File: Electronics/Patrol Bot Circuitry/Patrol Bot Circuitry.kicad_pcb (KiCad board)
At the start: 2 copper layers, 101 x 89.5 mm, 49 parts, among them J1 Left_Motor, J2 Right_Motor, J3 Battery, J4 AC_DC_10V, J5 Servo Motor, Q1 IRF4905, Q2 IRF4905, Q3 IRF4905, Q4 IRLZ44N, Q5 IRF4905, U1 ROB-14450, U10 HC-SR04, U11 MPU-6050, U2 ADS1115, U3 MP1584EN, U4 ESP32-CAM, U5 LM2931-3.3_TO220, U6 MAX9814, U7 MCP23017-E_SP, U8 HC-SR04, U9 HC-SR04

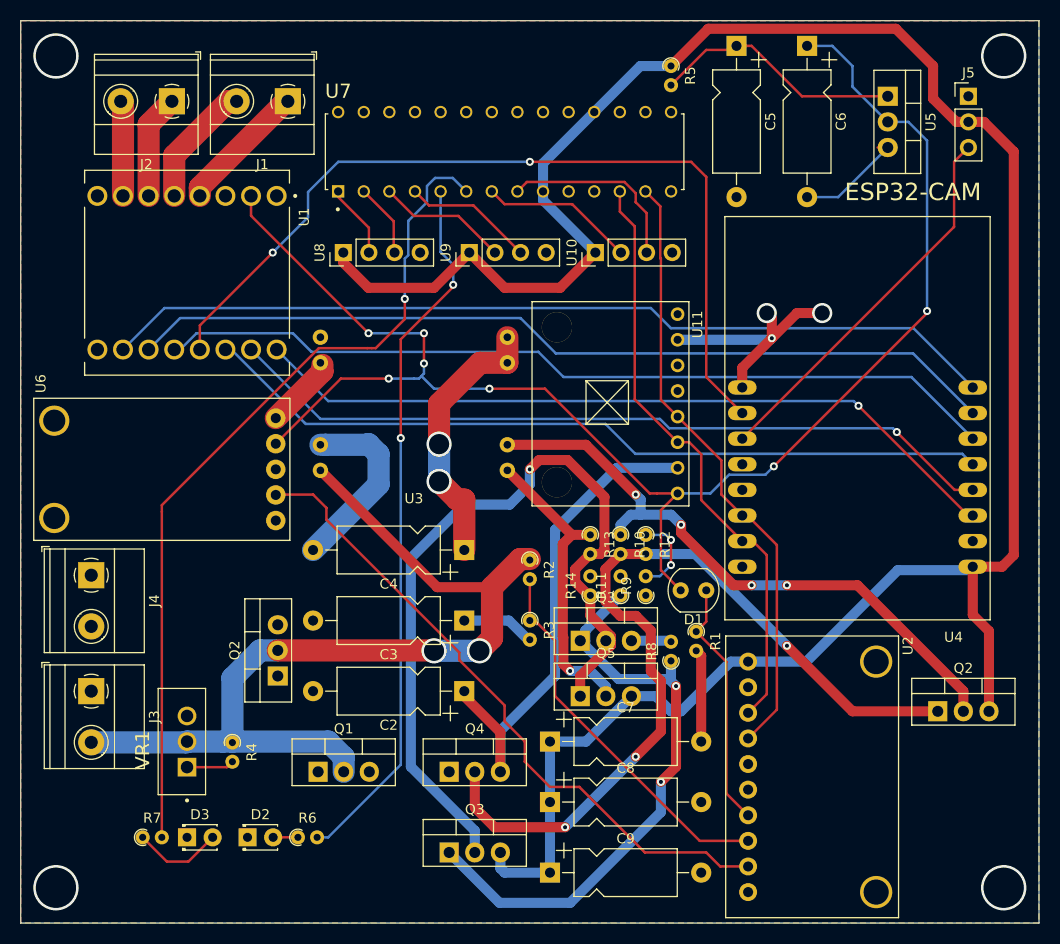
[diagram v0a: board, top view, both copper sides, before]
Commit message: Redesigned PCB / Mechanical Drawing
ESP32-cam not connecting to Wifi -> must DEBUG
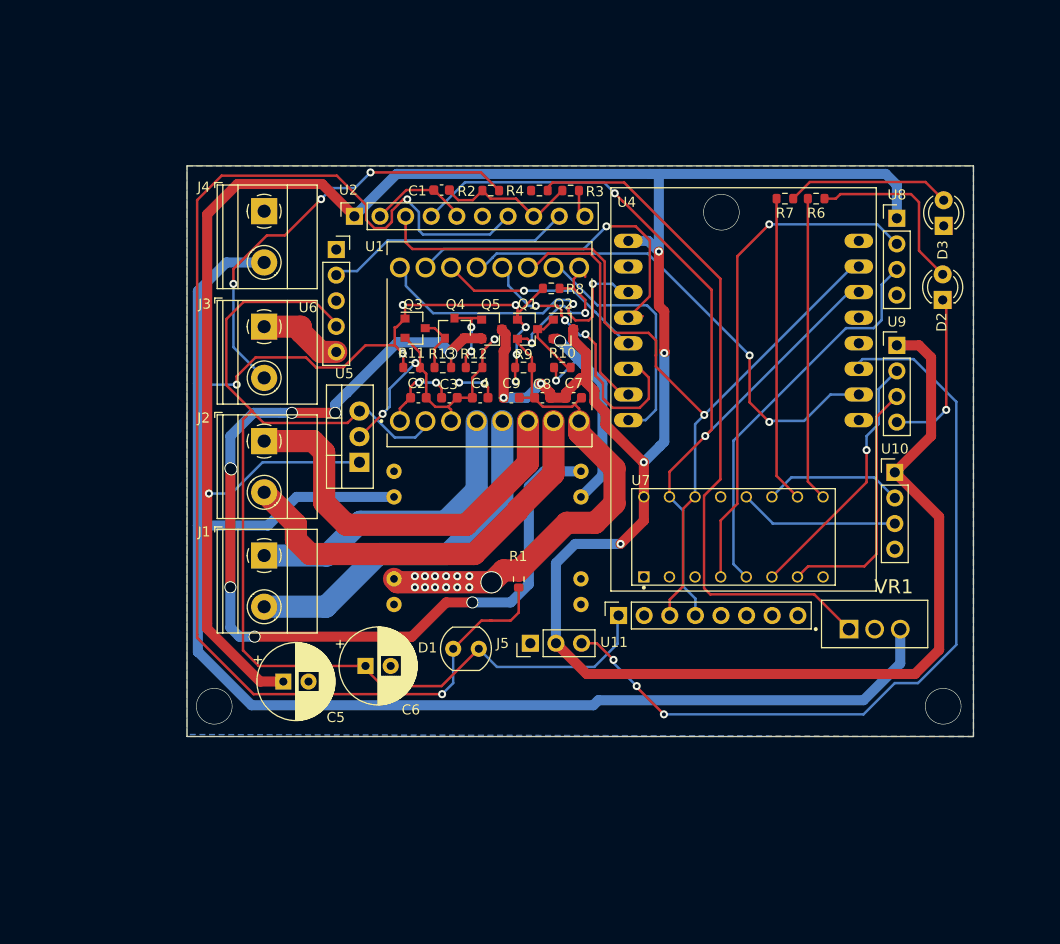
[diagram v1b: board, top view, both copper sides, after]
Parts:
- removed the Q2 at (182.5, 132.5)
- removed the Q2 at (117.0, 129.0)
- removed the Q3 at (147.0, 125.5)
- removed the Q3 at (134.0, 146.5)
- removed R14: 100k, Resistor_THT:R_Axial_DIN0204_L3.6mm_D1.6mm_P1.90mm_Vertical
- removed R5: 30, Resistor_THT:R_Axial_DIN0204_L3.6mm_D1.6mm_P1.90mm_Vertical
- added C1: 0.47u, Capacitor_SMD:C_0603_1608Metric, F.Cu at (133.2, 80.8)
- added Q2: Q_PMOS_GSD, Package_TO_SOT_SMD:SOT-23, F.Cu at (145.3, 94.6)
- added Q3: Q_NMOS_GSD, Package_TO_SOT_SMD:SOT-23, F.Cu at (130.6, 94.5)
- C2: value 20n -> 0.01n; footprint Capacitor_THT:CP_Axial_L10.0mm_D4.5mm_P15.00mm_Horizontal -> Capacitor_SMD:C_0603_1608Metric
- C3, C8: value 20n -> 0.1u; footprint Capacitor_THT:CP_Axial_L10.0mm_D4.5mm_P15.00mm_Horizontal -> Capacitor_SMD:C_0603_1608Metric
- C4, C7: value 20n -> 0.47u; footprint Capacitor_THT:CP_Axial_L10.0mm_D4.5mm_P15.00mm_Horizontal -> Capacitor_SMD:C_0603_1608Metric
- C5, C6: footprint Capacitor_THT:CP_Axial_L10.0mm_D4.5mm_P15.00mm_Horizontal -> Capacitor_THT:CP_Radial_D7.5mm_P2.50mm
- C9: value 20n -> 0.01u; footprint Capacitor_THT:CP_Axial_L10.0mm_D4.5mm_P15.00mm_Horizontal -> Capacitor_SMD:C_0603_1608Metric
- D2, D3: footprint LED_THT:LED_D1.8mm_W3.3mm_H2.4mm -> LED_THT:LED_D3.0mm
- Q1: value IRF4905 -> Q_NMOS_GSD; footprint Package_TO_SOT_THT:TO-220-3_Vertical -> Package_TO_SOT_SMD:SOT-23
- Q4: value IRLZ44N -> Q_PMOS_GSD; footprint Package_TO_SOT_THT:TO-220-3_Vertical -> Package_TO_SOT_SMD:SOT-23
- Q5: value IRF4905 -> Q_PMOS_GSD; footprint Package_TO_SOT_THT:TO-220-3_Vertical -> Package_TO_SOT_SMD:SOT-23
- R1: value 100K -> 200K; footprint Resistor_THT:R_Axial_DIN0204_L3.6mm_D1.6mm_P1.90mm_Vertical -> Resistor_SMD:R_0603_1608Metric
- R10, R11, R12, R13, R8, R9: value 100k -> 200k; footprint Resistor_THT:R_Axial_DIN0204_L3.6mm_D1.6mm_P1.90mm_Vertical -> Resistor_SMD:R_0603_1608Metric
- R2: value 600K -> 620K; footprint Resistor_THT:R_Axial_DIN0204_L3.6mm_D1.6mm_P1.90mm_Vertical -> Resistor_SMD:R_0603_1608Metric
- R3, R4, R6, R7: footprint Resistor_THT:R_Axial_DIN0204_L3.6mm_D1.6mm_P1.90mm_Vertical -> Resistor_SMD:R_0603_1608Metric
- U11: footprint MPU-6050:QFN50P400X400X95-24N -> Connector_PinSocket_2.54mm:PinSocket_1x08_P2.54mm_Vertical
- U2: footprint ADS1115:ADS1115 -> Connector_PinSocket_2.54mm:PinSocket_1x10_P2.54mm_Vertical
- U3: moved to B.Cu
- U6: footprint MAX9814:MAX9814 -> Connector_PinSocket_2.54mm:PinSocket_1x05_P2.54mm_Vertical
- U7: value MCP23017-E_SP -> PCF8574; footprint MCP23017:DIP787W45P254L3556H508Q28 -> PCF8574N:DIP794W45P254L1969H508Q16
- moved D3 96.5 mm to (183.1, 84.3), turned to 90 degrees
- moved R7 89.8 mm to (167.3, 81.7), turned to 180 degrees
- moved D2 87.1 mm to (182.9, 91.7), turned to 90 degrees
- moved R6 81.6 mm to (170.4, 81.7), turned to 180 degrees
- moved C5 77.4 mm to (117.5, 129.6), turned to 0 degrees
- moved C6 75.5 mm to (125.7, 128.0), turned to 0 degrees
- moved U2 71.8 mm to (124.6, 83.4), turned to 90 degrees
- moved J5 69.5 mm to (142.1, 125.8), turned to 90 degrees
- moved VR1 69.1 mm to (176.2, 124.3), turned to 0 degrees
- moved U5 63.7 mm to (125.1, 107.8), turned to 90 degrees
- moved R4 62.6 mm to (142.9, 80.8), turned to 0 degrees
- moved U8 55.0 mm to (178.4, 83.6), turned to 0 degrees
- moved Q1 48.6 mm to (141.8, 94.6)
- moved C9 47.3 mm to (140.2, 101.4)
- moved J1 45.1 mm to (115.7, 117.0), turned to 270 degrees
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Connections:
- C2 pad 2: +10V -> /Battery
- C3 pad 2: +10V -> /Battery
- C4 pad 2: +10V -> /Battery
- C5 pad 1: Net-(C5-Pad1) -> +5V
- C7 pad 1: /5V -> +5V
- C8 pad 1: /5V -> +5V
- C9 pad 1: /5V -> +5V
- J5 pad 2: /5V -> +5V
- Q1 pad 2: /Battery -> GND
- Q1 pad 3: +10V -> Net-(Q1-Pad3)
- Q4 pad 1: +10V -> Net-(Q3-Pad3)
- Q4 pad 2: Net-(Q2-Pad1) -> Net-(Q4-Pad2)
- Q4 pad 3: GND -> Net-(Q4-Pad3)
- Q5 pad 1: Net-(Q3-Pad2) -> Net-(Q4-Pad3)
- Q5 pad 2: Net-(Q5-Pad2) -> Net-(Q4-Pad2)
- Q5 pad 3: /5V -> +5V
- R10 pad 2: Net-(Q2-Pad1) -> Net-(Q1-Pad3)
- R12 pad 1: GND -> Net-(Q4-Pad3)
- R12 pad 2: Net-(Q2-Pad1) -> GND
- R13 pad 1: Net-(Q5-Pad2) -> Net-(Q4-Pad2)
- R13 pad 2: Net-(Q3-Pad2) -> Net-(Q3-Pad3)
- U1 pad 1: +10V -> /Battery
- U10 pad 1: /5V -> +5V
- U11 pad 7: Net-(U11-Pad7) -> GND
- U2 pad 1: /5V -> +5V
- U3 pad 1: Net-(Q5-Pad2) -> Net-(Q4-Pad2)
- U4 pad P$1: /5V -> +5V
- U5 pad 1: Net-(C5-Pad1) -> +5V
- U7 pad 1: Net-(U7-Pad1) -> GND
- U7 pad 10: GND -> Net-(R7-Pad2)
- U7 pad 11: (no net) -> Net-(U10-Pad2)
- U7 pad 12: /SCL -> Net-(U10-Pad3)
- U7 pad 13: /SDA -> Net-(U7-Pad13)
- U7 pad 14: (no net) -> /SCL
- U7 pad 15: GND -> /SDA
- U7 pad 16: GND -> +5V
- U7 pad 2: Net-(U7-Pad2) -> GND
- U7 pad 3: Net-(U7-Pad3) -> GND
- U7 pad 5: Net-(R6-Pad2) -> Net-(U7-Pad5)
- U7 pad 6: Net-(R7-Pad2) -> Net-(U7-Pad6)
- U7 pad 7: Net-(U10-Pad2) -> Net-(U7-Pad7)
- U7 pad 8: Net-(U10-Pad3) -> GND
- U7 pad 9: /5V -> Net-(R6-Pad2)
- U8 pad 1: /5V -> +5V
- U8 pad 2: Net-(U7-Pad1) -> Net-(U7-Pad4)
- U8 pad 3: Net-(U7-Pad2) -> Net-(U7-Pad5)
- U9 pad 1: /5V -> +5V
- U9 pad 2: Net-(U7-Pad3) -> Net-(U7-Pad6)
- U9 pad 3: Net-(U7-Pad4) -> Net-(U7-Pad7)
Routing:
- net +5V: track 0.00 -> 312.3 mm, vias 0 -> 7
- net /5V: track 231.1 -> 0.00 mm
- net +10V: track 77.3 -> 194.7 mm, vias 2 -> 7
- net Net-(D1-Pad1): track 24.9 -> 125.6 mm, vias 0 -> 2
- net Net-(Q4-Pad2): track 0.00 -> 98.3 mm, vias 0 -> 8
- net Net-(Q2-Pad1): track 86.1 -> 0.00 mm, vias 3 -> 0
- net Net-(Q3-Pad2): track 81.8 -> 0.00 mm, vias 1 -> 0
- net Net-(U1-Pad11): track 86.9 -> 21.5 mm
- net Net-(U1-Pad10): track 89.3 -> 24.6 mm
- net Net-(R4-Pad2): track 4.72 -> 69.0 mm
- net Net-(U1-Pad14): track 78.8 -> 20.7 mm, vias 0 -> 1
- net Net-(U1-Pad12): track 84.2 -> 30.6 mm, vias 0 -> 3
- net Net-(R7-Pad2): track 83.6 -> 30.4 mm, vias 1 -> 0
- net Net-(U1-Pad16): track 75.9 -> 30.8 mm, vias 1 -> 2
- net Net-(U1-Pad15): track 77.3 -> 35.2 mm
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- added copper zone on F.Cu, net /Battery
- removed copper zone on F.Cu, net +10V
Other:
- board size 101 x 89.5 mm -> 78 x 56.6 mm
